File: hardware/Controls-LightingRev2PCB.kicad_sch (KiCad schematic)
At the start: 33 parts, among them IC3 ACS724LLCTR-05AU-T, IC4 ACS724LLCTR-05AU-T, IC5 TLV70433DBVT, IC6 ACS724LLCTR-05AU-T, J1 53307-2471, J3 Conn_02x05_Top_Bottom, J4 Conn_01x02, J5 Conn_01x02, J6 Conn_01x03, Q3 IRLML0030, Q5 IRLML0030, U5 SN74LV1T34DBV

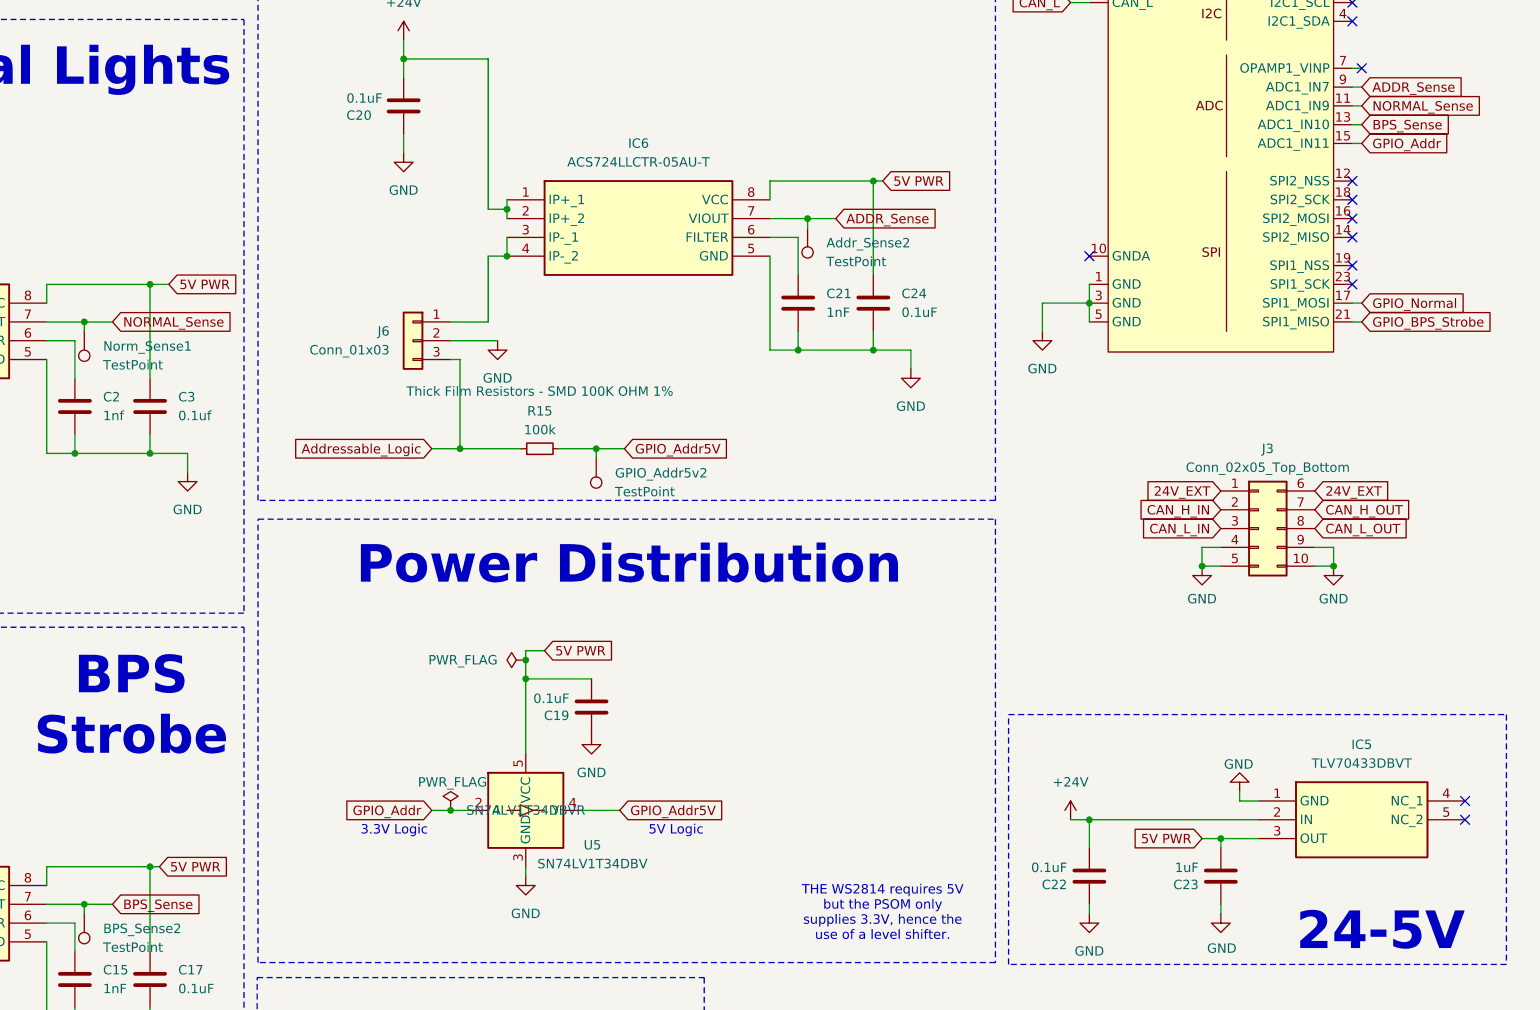
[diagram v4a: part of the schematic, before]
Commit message: Layout Review
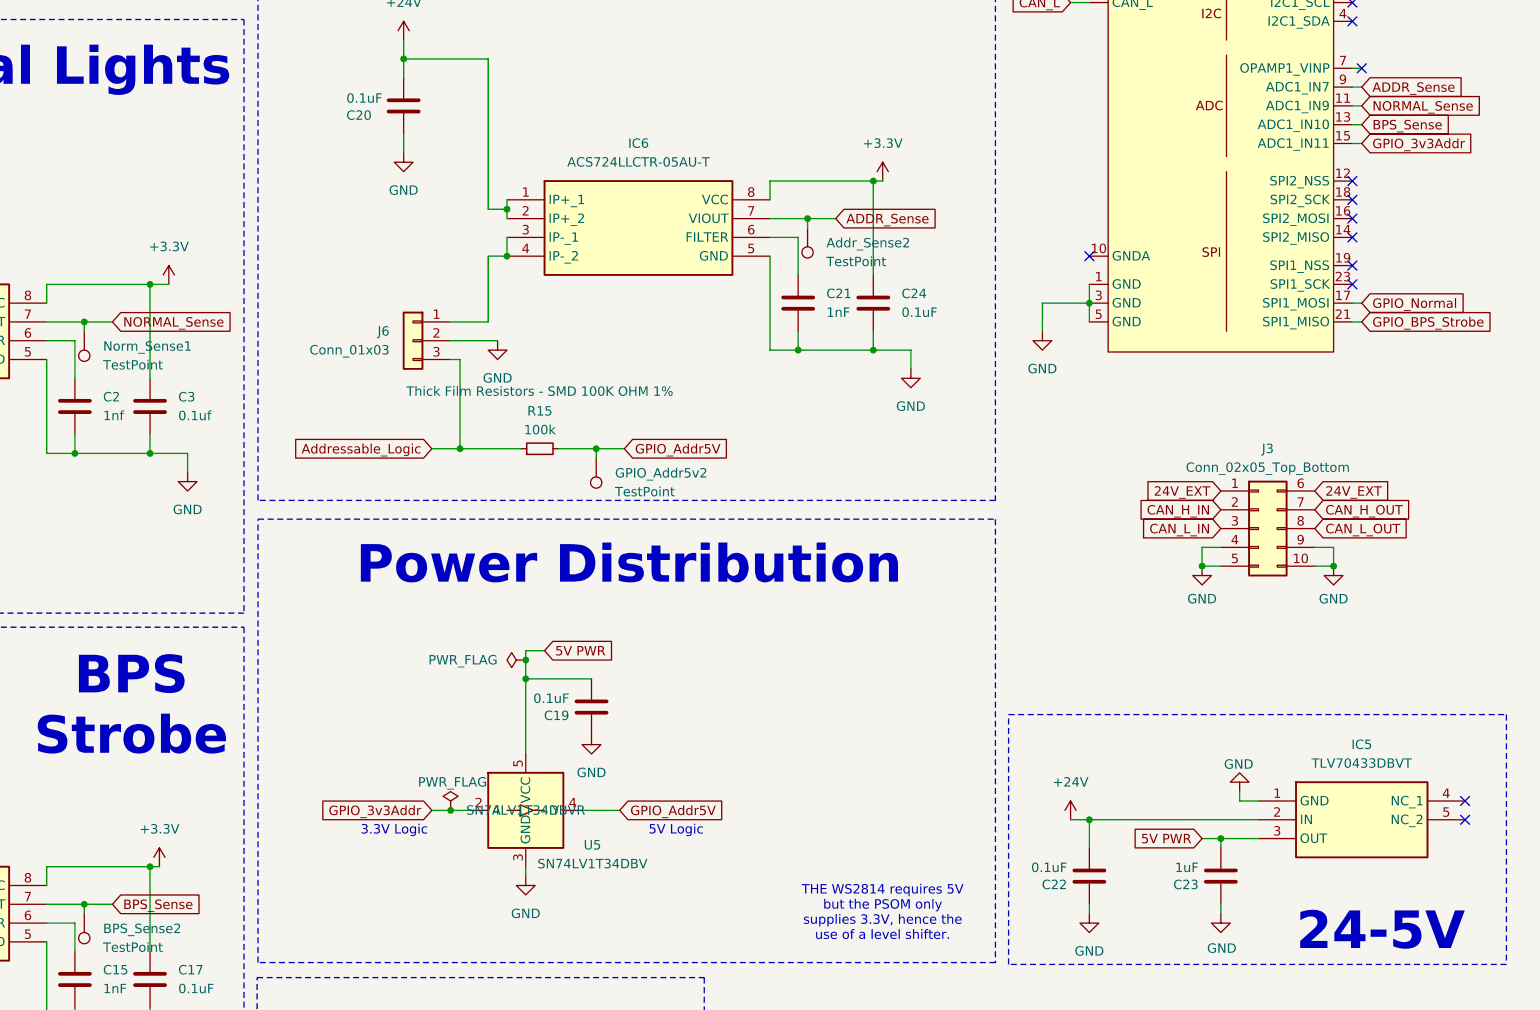
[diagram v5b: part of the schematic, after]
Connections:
- net +3.3V: now also C17.1, C24.1, C3.1, IC3.8 (VCC), IC4.8 (VCC), IC6.8 (VCC)
- net 5V PWR: no longer C17.1, C24.1, C3.1, IC3.8 (VCC), IC4.8 (VCC), IC6.8 (VCC)
- net GPIO_Addr renamed GPIO_3v3Addr
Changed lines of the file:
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@@
 		)
 	)
-	(global_label "GPIO_Addr"
+	(global_label "GPIO_3v3Addr"
 		(shape input)
 		(at 138.43 143.51 180)
@@
 		)
 		(property "Intersheetrefs" "${INTERSHEET_REFS}"
-			(at 125.8291 143.51 0)
+			(at 122.4425 143.51 0)
 			(effects
 				(font
@@
 		)
 	)
-	(global_label "5V PWR"
-		(shape input)
-		(at 101.6 151.13 0)
-		(fields_autoplaced yes)
-		(effects
-			(font
-				(size 1.27 1.27)
-			)
-			(justify left)
-		)
-		(property "Intersheetrefs" "${INTERSHEET_REFS}"
-			(at 111.8423 151.13 0)
-			(effects
-				(font
-					(size 1.27 1.27)
-				)
-				(justify left)
-				(hide yes)
-			)
-		)
-	)
 	(global_label "NORMAL_Sense"
 		(shape input)
@@
 		)
 	)
-	(global_label "GPIO_Addr"
+	(global_label "GPIO_3v3Addr"
 		(shape input)
 		(at 264.16 53.34 0)
@@
 		)
 		(property "Intersheetrefs" "${INTERSHEET_REFS}"
-			(at 276.7609 53.34 0)
+			(at 280.1475 53.34 0)
 			(effects
 				(font
@@
 		)
 	)
-	(global_label "5V PWR"
-		(shape input)
-		(at 102.87 72.39 0)
-		(fields_autoplaced yes)
-		(effects
-			(font
-				(size 1.27 1.27)
-			)
-			(justify left)
-		)
-		(property "Intersheetrefs" "${INTERSHEET_REFS}"
-			(at 113.1123 72.39 0)
-			(effects
-				(font
-					(size 1.27 1.27)
-				)
-				(justify left)
-				(hide yes)
-			)
-		)
-	)
 	(global_label "CAN_L_OUT"
 		(shape input)
@@
 		)
 	)
-	(global_label "5V PWR"
-		(shape input)
-		(at 199.39 58.42 0)
-		(fields_autoplaced yes)
-		(effects
-			(font
-				(size 1.27 1.27)
-			)
-			(justify left)
-		)
-		(property "Intersheetrefs" "${INTERSHEET_REFS}"
-			(at 209.6323 58.42 0)
-			(effects
-				(font
-					(size 1.27 1.27)
-				)
-				(justify left)
-				(hide yes)
-			)
-		)
-	)
 	(symbol
 		(lib_id "ACS724LLCTR:ACS724LLCTR-05AU-T")
@@
 	)
 	(symbol
+		(lib_id "power:+3.3V")
+		(at 199.39 58.42 0)
+		(unit 1)
+		(exclude_from_sim no)
+		(in_bom yes)
+		(on_board yes)
+		(dnp no)
+		(fields_autoplaced yes)
+		(property "Reference" "#PWR03"
+			(at 199.39 62.23 0)
+			(effects
+				(font
+					(size 1.27 1.27)
+				)
+				(hide yes)
+			)
+		)
+		(property "Value" "+3.3V"
+			(at 199.39 53.34 0)
+			(effects
+				(font
+					(size 1.27 1.27)
+				)
+			)
+		)
+		(property "Footprint" ""
+			(at 199.39 58.42 0)
+			(effects
+				(font
+					(size 1.27 1.27)
+				)
+				(hide yes)
+			)
+		)
+		(property "Datasheet" ""
+			(at 199.39 58.42 0)
+			(effects
+				(font
+					(size 1.27 1.27)
+				)
+				(hide yes)
+			)
+		)
+		(property "Description" "Power symbol creates a global label with name \"+3.3V\""
+			(at 199.39 58.42 0)
+			(effects
+				(font
+					(size 1.27 1.27)
+				)
+				(hide yes)
+			)
+		)
+		(pin "1"
+		)
+		(instances
+			(project "Controls-LightingRev2PCB"
+				(path "/4b4aadb4-8255-4dd1-afed-8a54e6d292d4"
+					(reference "#PWR03")
+					(unit 1)
+				)
+			)
+		)
+	)
+	(symbol
 		(lib_id "power:GND")
 		(at 260.35 110.49 0)
@@
 	)
 	(symbol
+		(lib_id "power:+3.3V")
+		(at 101.6 151.13 0)
+		(unit 1)
+		(exclude_from_sim no)
+		(in_bom yes)
+		(on_board yes)
+		(dnp no)
+		(fields_autoplaced yes)
+		(property "Reference" "#PWR010"
+			(at 101.6 154.94 0)
+			(effects
+				(font
+					(size 1.27 1.27)
+				)
+				(hide yes)
+			)
+		)
+		(property "Value" "+3.3V"
+			(at 101.6 146.05 0)
+			(effects
+				(font
+					(size 1.27 1.27)
+				)
+			)
+		)
+		(property "Footprint" ""
+			(at 101.6 151.13 0)
+			(effects
+				(font
+					(size 1.27 1.27)
+				)
+				(hide yes)
+			)
+		)
+		(property "Datasheet" ""
+			(at 101.6 151.13 0)
+			(effects
+				(font
+					(size 1.27 1.27)
+				)
+				(hide yes)
+			)
+		)
+		(property "Description" "Power symbol creates a global label with name \"+3.3V\""
+			(at 101.6 151.13 0)
+			(effects
+				(font
+					(size 1.27 1.27)
+				)
+				(hide yes)
+			)
+		)
+		(pin "1"
+		)
+		(instances
+			(project "Controls-LightingRev2PCB"
+				(path "/4b4aadb4-8255-4dd1-afed-8a54e6d292d4"
+					(reference "#PWR010")
+					(unit 1)
+				)
+			)
+		)
+	)
+	(symbol
 		(lib_id "power:PWR_FLAG")
 		(at 151.13 123.19 90)
@@
 					(unit 1)
 				)
+			)
+		)
+	)
+	(symbol
+		(lib_id "power:+3.3V")
+		(at 102.87 72.39 0)
+		(unit 1)
+		(exclude_from_sim no)
+		(in_bom yes)
+		(on_board yes)
+		(dnp no)
+		(fields_autoplaced yes)
+		(property "Reference" "#PWR09"
+			(at 102.87 76.2 0)
+			(effects
+				(font
+					(size 1.27 1.27)
+				)
+				(hide yes)
+			)
+		)
+		(property "Value" "+3.3V"
+			(at 102.87 67.31 0)
+			(effects
+				(font
+					(size 1.27 1.27)
+				)
+			)
+		)
+		(property "Footprint" ""
+			(at 102.87 72.39 0)
+			(effects
+				(font
+					(size 1.27 1.27)
+				)
+				(hide yes)
+			)
+		)
+		(property "Datasheet" ""
+			(at 102.87 72.39 0)
+			(effects
+				(font
+					(size 1.27 1.27)
+				)
+				(hide yes)
+			)
+		)
+		(property "Description" "Power symbol creates a global label with name \"+3.3V\""
+			(at 102.87 72.39 0)
+			(effects
+				(font
+					(size 1.27 1.27)
+				)
+				(hide yes)
+			)
+		)
+		(pin "1"
+		)
+		(instances
+			(project "Controls-LightingRev2PCB"
+				(path "/4b4aadb4-8255-4dd1-afed-8a54e6d292d4"
+					(reference "#PWR09")
+					(unit 1)
+				)

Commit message: All review requests escept LDO addressed
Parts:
- Addr_Sense2, BPS_Sense2, GPIO_Addr5v2, GPIO_BPS2, GPIO_Norm1, Norm_Sense1: footprint UTSVT_Special:TestPoint_HEX_3mmID -> TestPoint:TestPoint_Keystone_5005-5009_Compact
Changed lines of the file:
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@@
 			)
 		)
-		(property "Footprint" "UTSVT_Special:TestPoint_HEX_3mmID"
+		(property "Footprint" "TestPoint:TestPoint_Keystone_5005-5009_Compact"
 			(at 40.64 175.26 0)
 			(effects
@@
 			)
 		)
-		(property "Footprint" "UTSVT_Special:TestPoint_HEX_3mmID"
+		(property "Footprint" "TestPoint:TestPoint_Keystone_5005-5009_Compact"
 			(at 39.37 96.52 0)
 			(effects
@@
 			)
 		)
-		(property "Footprint" "UTSVT_Special:TestPoint_HEX_3mmID"
+		(property "Footprint" "TestPoint:TestPoint_Keystone_5005-5009_Compact"
 			(at 86.36 157.48 0)
 			(effects
@@
 			)
 		)
-		(property "Footprint" "UTSVT_Special:TestPoint_HEX_3mmID"
+		(property "Footprint" "TestPoint:TestPoint_Keystone_5005-5009_Compact"
 			(at 184.15 64.77 0)
 			(effects
@@
 			)
 		)
-		(property "Footprint" "UTSVT_Special:TestPoint_HEX_3mmID"
+		(property "Footprint" "TestPoint:TestPoint_Keystone_5005-5009_Compact"
 			(at 86.36 78.74 0)
 			(effects
@@
 			)
 		)
-		(property "Footprint" "UTSVT_Special:TestPoint_HEX_3mmID"
+		(property "Footprint" "TestPoint:TestPoint_Keystone_5005-5009_Compact"
 			(at 155.575 95.885 0)
 			(effects

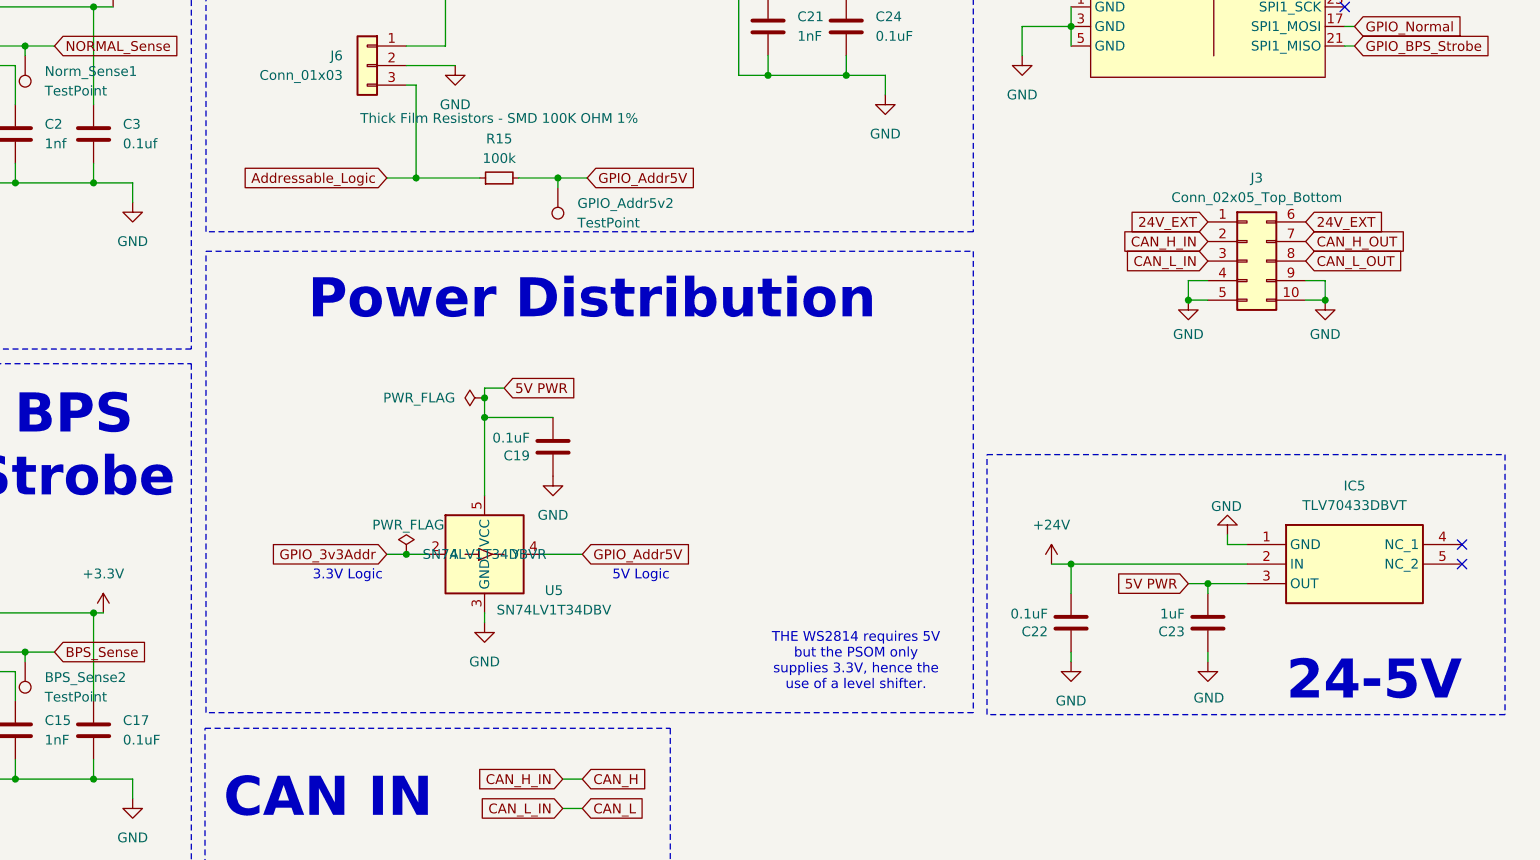
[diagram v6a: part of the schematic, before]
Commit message: Changes from Review Request
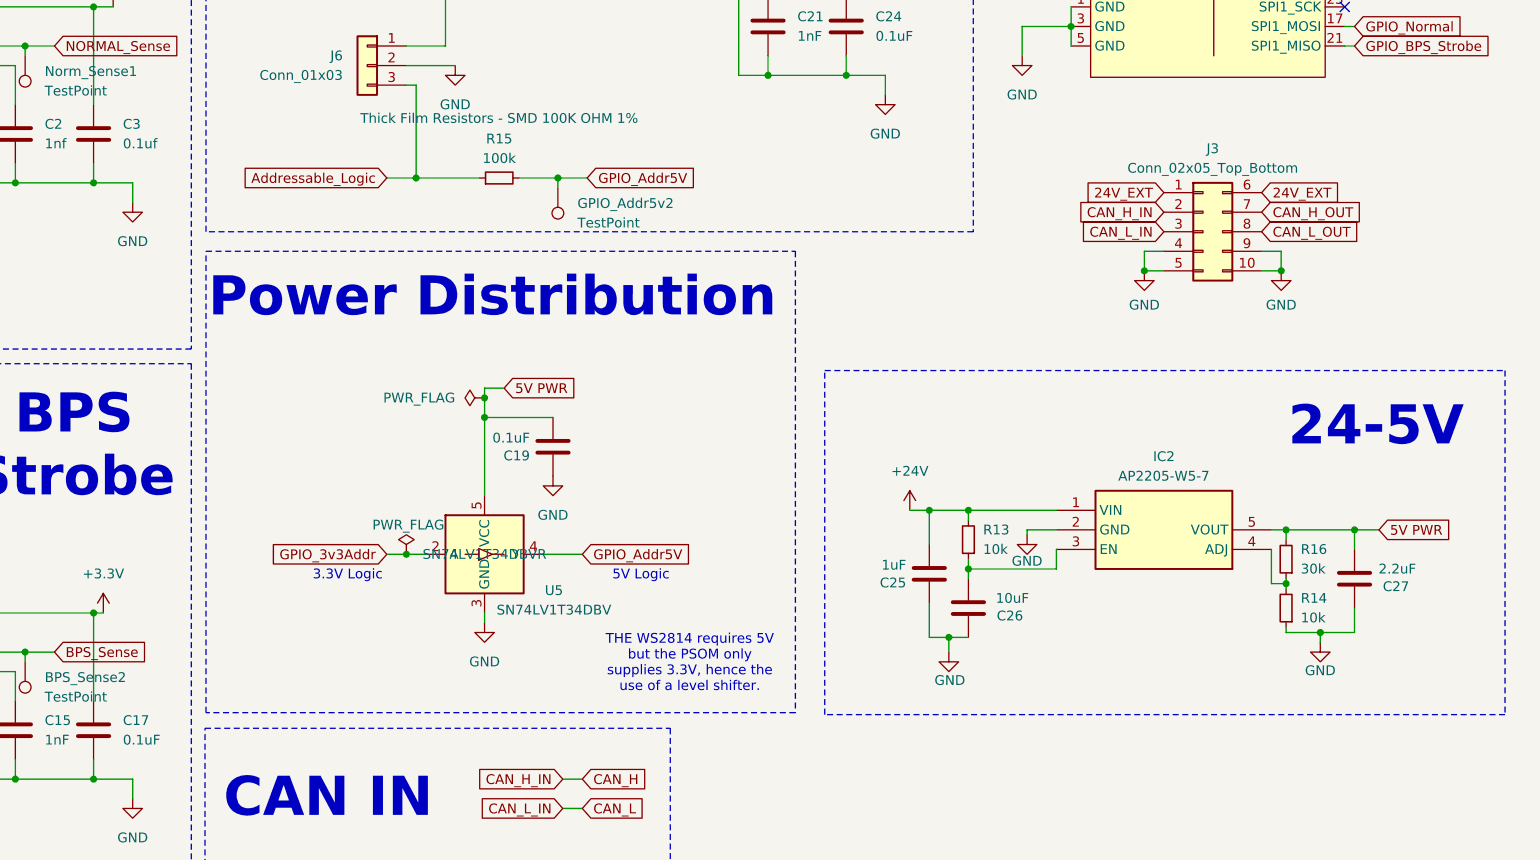
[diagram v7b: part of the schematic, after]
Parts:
- removed C22: 0.1uF, Capacitor_SMD:C_0603_1608Metric, symbol Device:C
- removed C23: 1uF, Capacitor_SMD:C_0603_1608Metric, symbol Device:C
- removed IC5: TLV70433DBVT, Lighting_Board:SOT95P280X145-5N, symbol TLB70433DBVT:TLV70433DBVT
- added C25: 1uF, Capacitor_SMD:C_0603_1608Metric, symbol Device:C
- added C26: 10uF, Capacitor_SMD:C_0603_1608Metric, symbol Device:C
- added C27: 2.2uF, Capacitor_SMD:C_0603_1608Metric, symbol Device:C
- added IC2: AP2205-W5-7, AP2205W57, symbol 24-5-LDO:AP2205-W5-7
- added R13, R14: 10k, Resistor_SMD:R_0603_1608Metric, symbol Device:R_Small
- added R16: 30k, Resistor_SMD:R_0603_1608Metric, symbol Device:R_Small
- Addr_Sense2, BPS_Sense2, GPIO_Addr5v2, GPIO_BPS2, GPIO_Norm1, Norm_Sense1: footprint TestPoint:TestPoint_Keystone_5005-5009_Compact -> UTSVT_Special:TestPoint_HEX_3mmID
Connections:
- net +24V: now also C25.2, IC2.1 (VIN), R13.2
- net 5V PWR: now also C27.2, IC2.5 (VOUT), R16.2
- net GND: now also C25.1, C26.1, C27.1, IC2.2 (GND), R14.1
- new net: C26.2, IC2.3 (EN), R13.1
- new net: IC2.4 (ADJ), R14.2, R16.1
- no-connect marks 13 -> 11
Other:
- moved on the sheet: J3

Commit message: Layout complete and ready for review
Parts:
- Addr_Sense2, BPS_Sense2, GPIO_Addr5v2, GPIO_BPS2, GPIO_Norm1, Norm_Sense1: footprint UTSVT_Special:TestPoint_HEX_3mmID -> TestPoint:TestPoint_Keystone_5005-5009_Compact
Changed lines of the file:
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@@
 			)
 		)
-		(property "Footprint" "UTSVT_Special:TestPoint_HEX_3mmID"
+		(property "Footprint" "TestPoint:TestPoint_Keystone_5005-5009_Compact"
 			(at 40.64 175.26 0)
 			(effects
@@
 			)
 		)
-		(property "Footprint" "UTSVT_Special:TestPoint_HEX_3mmID"
+		(property "Footprint" "TestPoint:TestPoint_Keystone_5005-5009_Compact"
 			(at 39.37 96.52 0)
 			(effects
@@
 			)
 		)
-		(property "Footprint" "UTSVT_Special:TestPoint_HEX_3mmID"
+		(property "Footprint" "TestPoint:TestPoint_Keystone_5005-5009_Compact"
 			(at 86.36 157.48 0)
 			(effects
@@
 			)
 		)
-		(property "Footprint" "UTSVT_Special:TestPoint_HEX_3mmID"
+		(property "Footprint" "TestPoint:TestPoint_Keystone_5005-5009_Compact"
 			(at 184.15 64.77 0)
 			(effects
@@
 			)
 		)
-		(property "Footprint" "UTSVT_Special:TestPoint_HEX_3mmID"
+		(property "Footprint" "TestPoint:TestPoint_Keystone_5005-5009_Compact"
 			(at 86.36 78.74 0)
 			(effects
@@
 			)
 		)
-		(property "Footprint" "UTSVT_Special:TestPoint_HEX_3mmID"
+		(property "Footprint" "TestPoint:TestPoint_Keystone_5005-5009_Compact"
 			(at 155.575 95.885 0)
 			(effects
